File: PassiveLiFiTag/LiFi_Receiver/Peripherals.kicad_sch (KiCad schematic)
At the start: 4 parts, among them J1 Conn_01x07, SW1 SW_Push

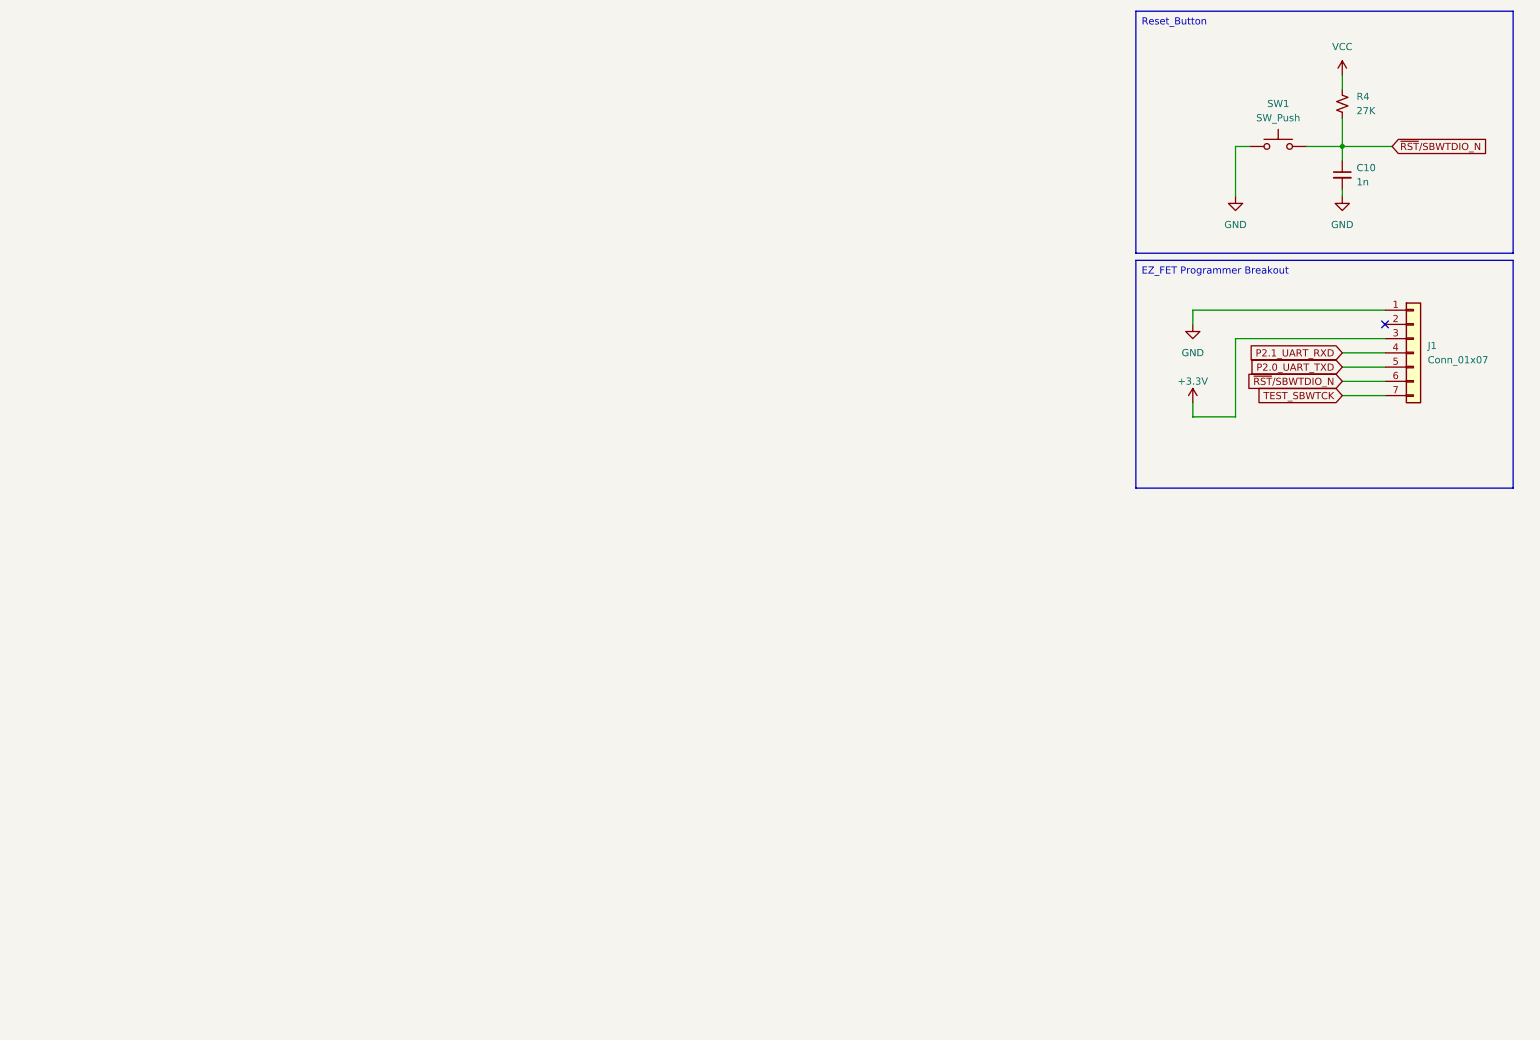
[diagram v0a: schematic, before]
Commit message: Added Updates
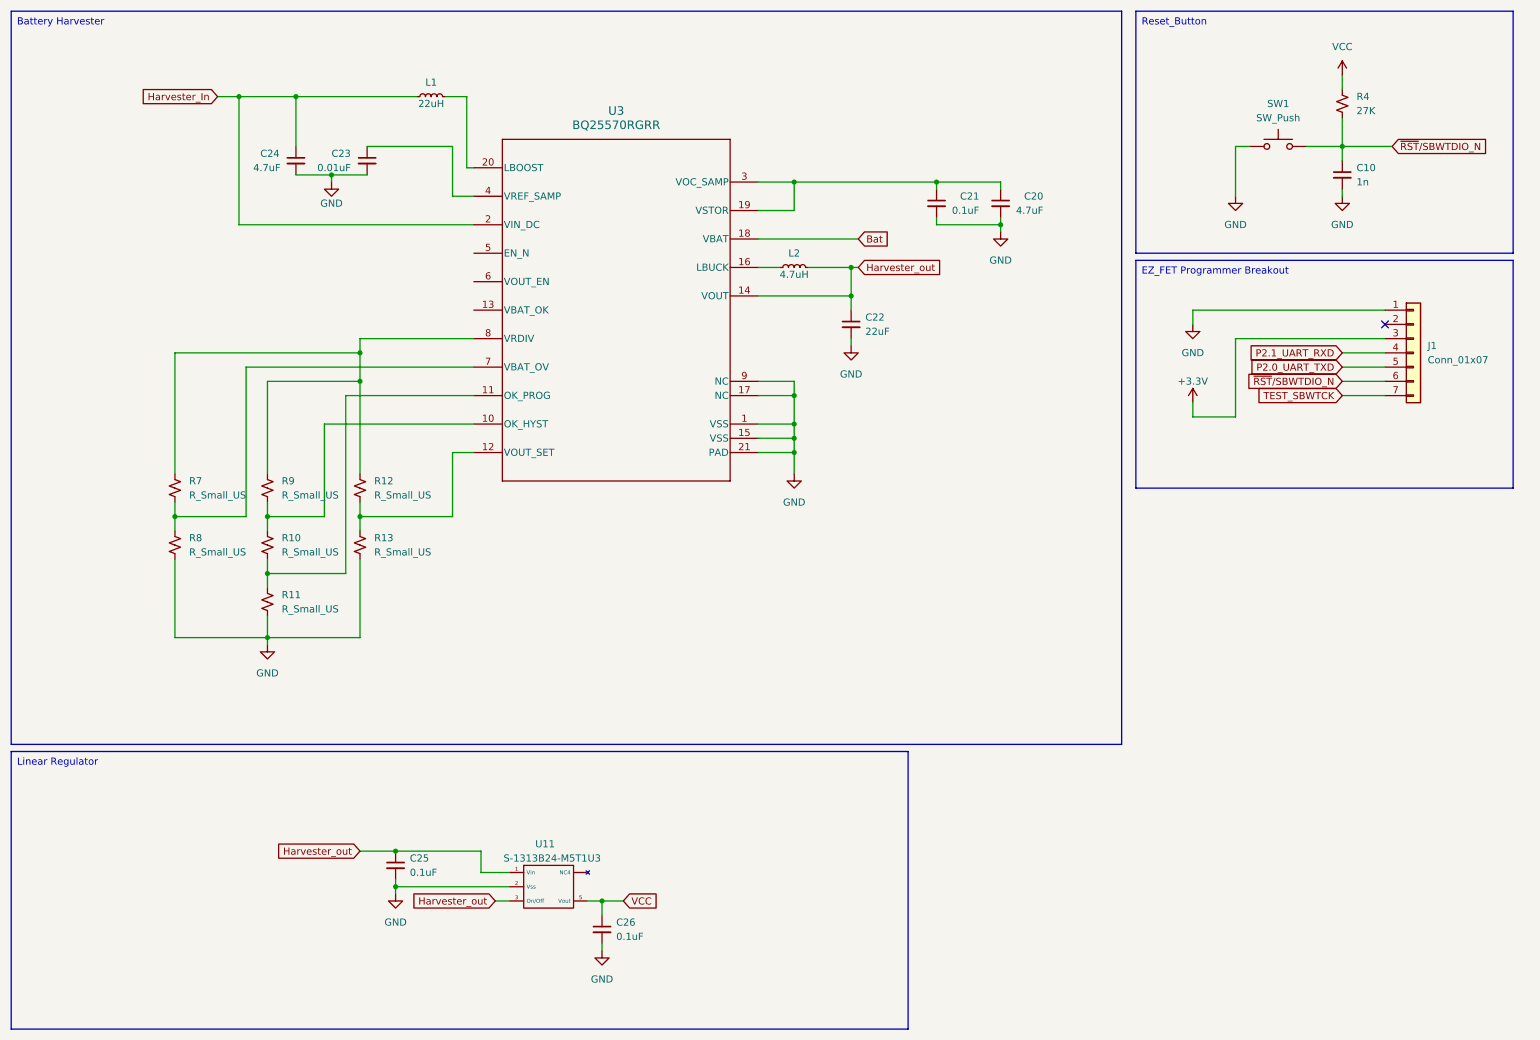
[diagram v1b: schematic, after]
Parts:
- added C20, C24: 4.7uF, Capacitor_SMD:C_01005_0402Metric, symbol Device:C_Small
- added C21, C25, C26: 0.1uF, Capacitor_SMD:C_01005_0402Metric, symbol Device:C_Small
- added C22: 22uF, Capacitor_SMD:C_01005_0402Metric, symbol Device:C_Small
- added C23: 0.01uF, Capacitor_SMD:C_01005_0402Metric, symbol Device:C_Small
- added L1: 22uH, Inductor_SMD:L_01005_0402Metric, symbol Device:L_Small
- added L2: 4.7uH, Inductor_SMD:L_01005_0402Metric, symbol Device:L_Small
- added R10, R11, R12, R13, R7, R8, R9: R_Small_US, Resistor_SMD:R_01005_0402Metric, symbol Device:R_Small_US
- added U11: S-1313B24-M5T1U3, Package_TO_SOT_SMD:SOT-23-5, symbol LifiLib:S-1313B24-M5T1U3
- added U3: BQ25570RGRR, Library:Bat_Harv2, symbol LiFi_Receiver:BQ25570RGRR
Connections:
- net GND: now also C20.2, C21.2, C22.2, C23.2, C24.2, C25.2, C26.2, R11.2, R13.2, R8.2, U11.2 (Vss), U3.1 (VSS), U3.15 (VSS), U3.17 (NC), U3.21 (PAD), U3.9 (NC)
- net VCC: now also C26.1, U11.5 (Vout)
- new net: R7.2, R8.1, U3.7 (VBAT_OV)
- new net: L2.2, U3.16 (LBUCK)
- new net: R10.2, R11.1, U3.11 (OK_PROG)
- new net: R12.1, R7.1, R9.1, U3.8 (VRDIV)
- new net: R12.2, R13.1, U3.12 (VOUT_SET)
- new net: C20.1, C21.1, U3.19 (VSTOR), U3.3 (VOC_SAMP)
- new net: L1.1, U3.20 (LBOOST)
- new net: C23.1, U3.4 (VREF_SAMP)
- new net: R10.1, R9.2, U3.10 (OK_HYST)
- new net Bat: U3.18 (VBAT)
- new net Harvester_In: C24.1, L1.2, U3.2 (VIN_DC)
- new net Harvester_out: C22.1, C25.1, L2.1, U11.1 (Vin), U11.3 (On/Off), U3.14 (VOUT)
